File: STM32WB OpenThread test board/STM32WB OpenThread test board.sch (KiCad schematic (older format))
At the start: 15 parts

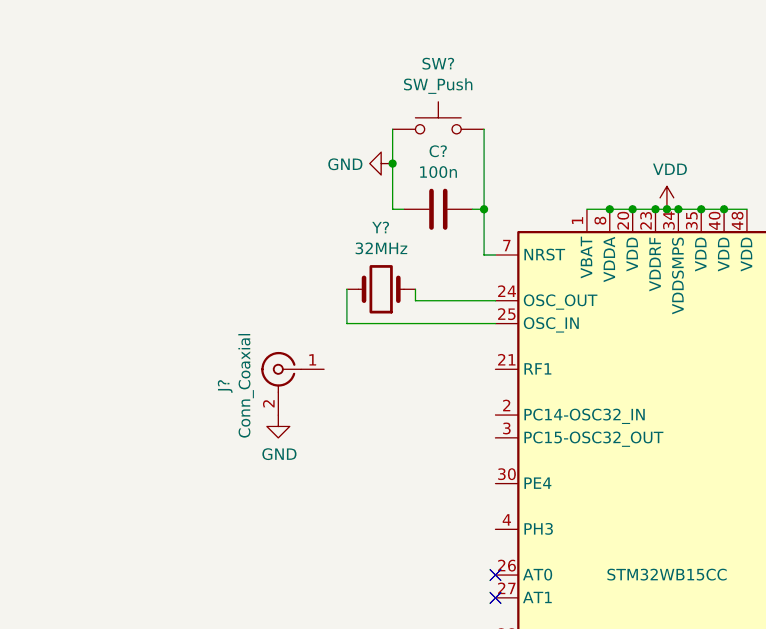
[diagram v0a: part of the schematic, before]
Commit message: WIP
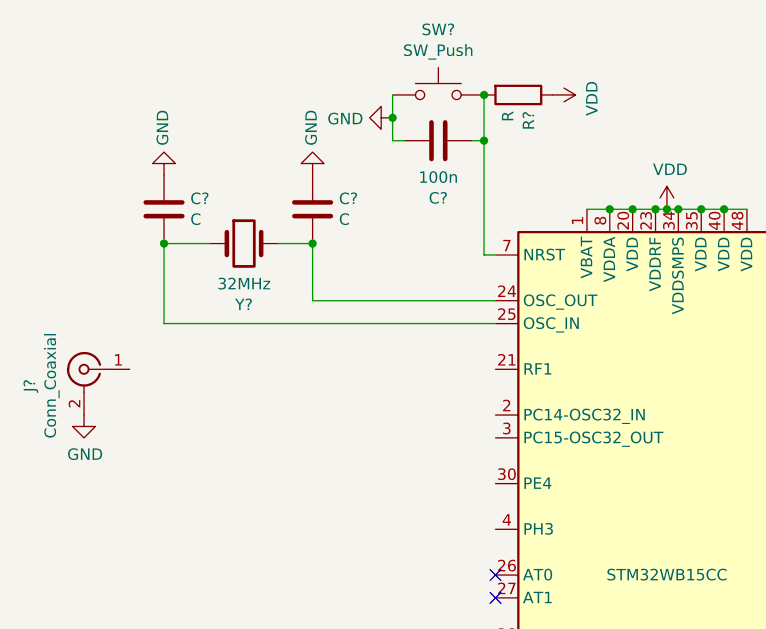
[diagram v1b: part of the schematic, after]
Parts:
- added C? (x2): C, symbol Device:C
- added R?: R, symbol Device:R
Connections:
- net GND: now also C?.1, C?.1, C?.1; no longer C?.2
- net VDD: now also R?.1
- net at U?.24 (OSC_OUT): now also Y?.2, C?.2; no longer Y?.1
- net at U?.25 (OSC_IN): now also Y?.1, C?.2; no longer Y?.2
- net at SW?.2, U?.7 (NRST): now also C?.2, R?.2; no longer C?.1
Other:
- moved on the sheet: C?, J?, SW?, Y?
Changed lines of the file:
@@
 L Device:Crystal Y?
 U 1 1 6229DF59
-P 4450 1750
-F 0 "Y?" H 4450 1482 50  0000 C CNN
-F 1 "32MHz" H 4450 1573 50  0000 C CNN
-F 2 "" H 4450 1750 50  0001 C CNN
-F 3 "~" H 4450 1750 50  0001 C CNN
-	1    4450 1750
-	-1   0    0    1
-$EndComp
-Wire Wire Line
-	4600 1800 4950 1800
-Wire Wire Line
-	4950 1900 4300 1900
-Wire Wire Line
-	4600 1800 4600 1750
-Wire Wire Line
-	4300 1750 4300 1900
+P 3850 1550
+F 0 "Y?" H 3850 1282 50  0000 C CNN
+F 1 "32MHz" H 3850 1373 50  0000 C CNN
+F 2 "" H 3850 1550 50  0001 C CNN
+F 3 "~" H 3850 1550 50  0001 C CNN
+	1    3850 1550
+	1    0    0    -1
+$EndComp
 Wire Wire Line
 	5350 1400 5450 1400
@@
 L Connector:Conn_Coaxial J?
 U 1 1 622A9FE4
-P 4000 2100
-F 0 "J?" V 4237 2029 50  0000 C CNN
-F 1 "Conn_Coaxial" V 4146 2029 50  0000 C CNN
-F 2 "" H 4000 2100 50  0001 C CNN
-F 3 " ~" H 4000 2100 50  0001 C CNN
-	1    4000 2100
+P 3150 2100
+F 0 "J?" V 3387 2029 50  0000 C CNN
+F 1 "Conn_Coaxial" V 3296 2029 50  0000 C CNN
+F 2 "" H 3150 2100 50  0001 C CNN
+F 3 " ~" H 3150 2100 50  0001 C CNN
+	1    3150 2100
 	-1   0    0    -1
 $EndComp
@@
 L power:GND #PWR?
 U 1 1 622AEBD7
-P 4000 2300
-F 0 "#PWR?" H 4000 2050 50  0001 C CNN
-F 1 "GND" H 4005 2127 50  0000 C CNN
-F 2 "" H 4000 2300 50  0001 C CNN
-F 3 "" H 4000 2300 50  0001 C CNN
-	1    4000 2300
+P 3150 2300
+F 0 "#PWR?" H 3150 2050 50  0001 C CNN
+F 1 "GND" H 3155 2127 50  0000 C CNN
+F 2 "" H 3150 2300 50  0001 C CNN
+F 3 "" H 3150 2300 50  0001 C CNN
+	1    3150 2300
 	1    0    0    -1
 $EndComp
@@
 L Switch:SW_Push SW?
 U 1 1 622BE53E
-P 4700 1050
-F 0 "SW?" H 4700 1335 50  0000 C CNN
-F 1 "SW_Push" H 4700 1244 50  0000 C CNN
-F 2 "" H 4700 1250 50  0001 C CNN
-F 3 "~" H 4700 1250 50  0001 C CNN
-	1    4700 1050
+P 4700 900
+F 0 "SW?" H 4700 1185 50  0000 C CNN
+F 1 "SW_Push" H 4700 1094 50  0000 C CNN
+F 2 "" H 4700 1100 50  0001 C CNN
+F 3 "~" H 4700 1100 50  0001 C CNN
+	1    4700 900
 	1    0    0    -1
 $EndComp
@@
 L power:GND #PWR?
 U 1 1 622BF9B2
-P 4500 1200
-F 0 "#PWR?" H 4500 950 50  0001 C CNN
-F 1 "GND" V 4505 1072 50  0000 R CNN
-F 2 "" H 4500 1200 50  0001 C CNN
-F 3 "" H 4500 1200 50  0001 C CNN
-	1    4500 1200
+P 4500 1000
+F 0 "#PWR?" H 4500 750 50  0001 C CNN
+F 1 "GND" V 4505 872 50  0000 R CNN
+F 2 "" H 4500 1000 50  0001 C CNN
+F 3 "" H 4500 1000 50  0001 C CNN
+	1    4500 1000
 	0    1    1    0
 $EndComp
-Wire Wire Line
-	4900 1050 4900 1400
+$Comp
+L Device:C C?
+U 1 1 622C3467
+P 4700 1100
+F 0 "C?" V 4448 1100 50  0000 C CNN
+F 1 "100n" V 4539 1100 50  0000 C CNN
+F 2 "" H 4738 950 50  0001 C CNN
+F 3 "~" H 4700 1100 50  0001 C CNN
+	1    4700 1100
+	0    -1   -1   0
+$EndComp
+$Comp
+L power:VDD #PWR?
+U 1 1 622E9133
+P 5200 900
+F 0 "#PWR?" H 5200 750 50  0001 C CNN
+F 1 "VDD" H 5215 1073 50  0000 C CNN
+F 2 "" H 5200 900 50  0001 C CNN
+F 3 "" H 5200 900 50  0001 C CNN
+	1    5200 900
+	0    1    1    0
+$EndComp
+$Comp
+L Device:R R?
+U 1 1 622E9FBF
+P 5050 900
+F 0 "R?" H 5120 946 50  0000 L CNN
+F 1 "R" H 5120 855 50  0000 L CNN
+F 2 "" V 4980 900 50  0001 C CNN
+F 3 "~" H 5050 900 50  0001 C CNN
+	1    5050 900
+	0    1    1    0
+$EndComp
+Wire Wire Line
+	4500 1000 4500 900
+Wire Wire Line
+	4500 1000 4500 1100
+Wire Wire Line
+	4500 1100 4550 1100
+Connection ~ 4500 1000
+Connection ~ 4900 900
+Wire Wire Line
+	4850 1100 4900 1100
+Wire Wire Line
+	4900 1100 4900 900
+Wire Wire Line
+	4900 1100 4900 1600
 Wire Wire Line
 	4900 1600 4950 1600
-$Comp
-L Device:C C?
-U 1 1 622C3467
-P 4700 1400
-F 0 "C?" V 4448 1400 50  0000 C CNN
-F 1 "100n" V 4539 1400 50  0000 C CNN
-F 2 "" H 4738 1250 50  0001 C CNN
-F 3 "~" H 4700 1400 50  0001 C CNN
-	1    4700 1400
-	0    1    1    0
-$EndComp
-Wire Wire Line
-	4850 1400 4900 1400
-Connection ~ 4900 1400
-Wire Wire Line
-	4900 1400 4900 1600
-Wire Wire Line
-	4500 1050 4500 1200
-Wire Wire Line
-	4500 1200 4500 1400
-Wire Wire Line
-	4500 1400 4550 1400
-Connection ~ 4500 1200
+Connection ~ 4900 1100
+$Comp
+L power:GND #PWR?
+U 1 1 62304964
+P 4150 1250
+F 0 "#PWR?" H 4150 1000 50  0001 C CNN
+F 1 "GND" V 4155 1122 50  0000 R CNN
+F 2 "" H 4150 1250 50  0001 C CNN
+F 3 "" H 4150 1250 50  0001 C CNN
+	1    4150 1250
+	-1   0    0    1
+$EndComp
+$Comp
+L power:GND #PWR?
+U 1 1 62304EE0
+P 3500 1250
+F 0 "#PWR?" H 3500 1000 50  0001 C CNN
+F 1 "GND" V 3505 1122 50  0000 R CNN
+F 2 "" H 3500 1250 50  0001 C CNN
+F 3 "" H 3500 1250 50  0001 C CNN
+	1    3500 1250
+	-1   0    0    1
+$EndComp
+Wire Wire Line
+	3700 1550 3500 1550
+Wire Wire Line
+	4000 1550 4150 1550
+$Comp
+L Device:C C?
+U 1 1 6230A174
+P 4150 1400
+F 0 "C?" H 4265 1446 50  0000 L CNN
+F 1 "C" H 4265 1355 50  0000 L CNN
+F 2 "" H 4188 1250 50  0001 C CNN
+F 3 "~" H 4150 1400 50  0001 C CNN
+	1    4150 1400
+	1    0    0    -1
+$EndComp
+$Comp
+L Device:C C?
+U 1 1 6230A550
+P 3500 1400
+F 0 "C?" H 3615 1446 50  0000 L CNN
+F 1 "C" H 3615 1355 50  0000 L CNN
+F 2 "" H 3538 1250 50  0001 C CNN
+F 3 "~" H 3500 1400 50  0001 C CNN
+	1    3500 1400
+	1    0    0    -1
+$EndComp
+Wire Wire Line
+	4950 1800 4150 1800
+Connection ~ 4150 1550
+Wire Wire Line
+	4950 1900 3500 1900
+Connection ~ 3500 1550
+Wire Wire Line
+	4150 1550 4150 1800
+Wire Wire Line
+	3500 1550 3500 1900
 $EndSCHEMATC
